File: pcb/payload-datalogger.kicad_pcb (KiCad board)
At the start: 2 copper layers, 43.5 x 41 mm, 42 parts, among them J1 2.54mm 01x02 header, J2 Conn_01x02, J3 Conn_01x02, J4 Conn_01x02, J5 Conn_01x02, SW2 PTS815, U1 XIAO-ESP32-C3-DIP, U2 NCP177AMX330TCG, U3 W25X40CLSN, U4 MCP96RL00T-E_MX, U5 MCP96RL00T-E_MX, U6 MCP96RL00T-E_MX, U7 MCP96RL00T-E_MX

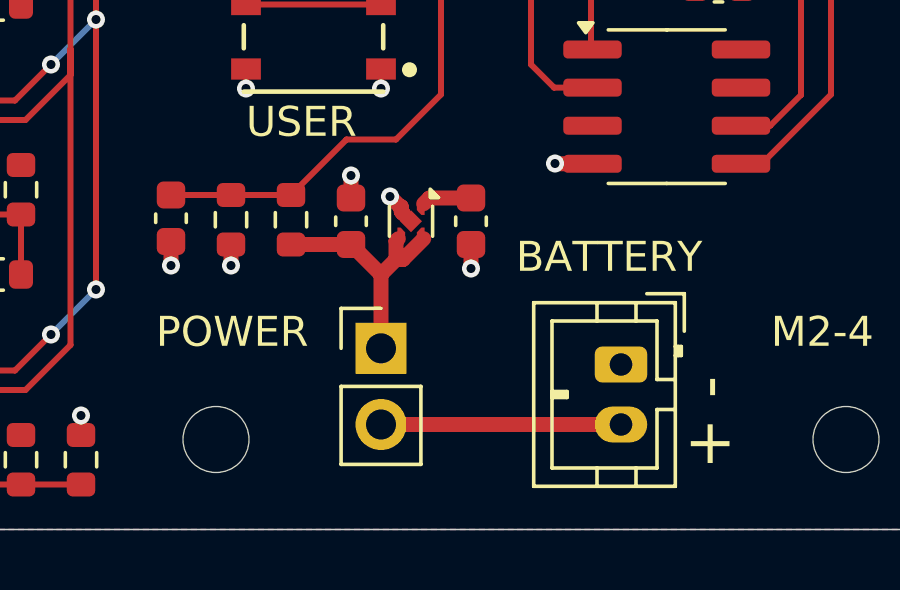
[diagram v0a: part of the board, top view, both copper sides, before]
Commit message: Update payload-datalogger.kicad_pcb
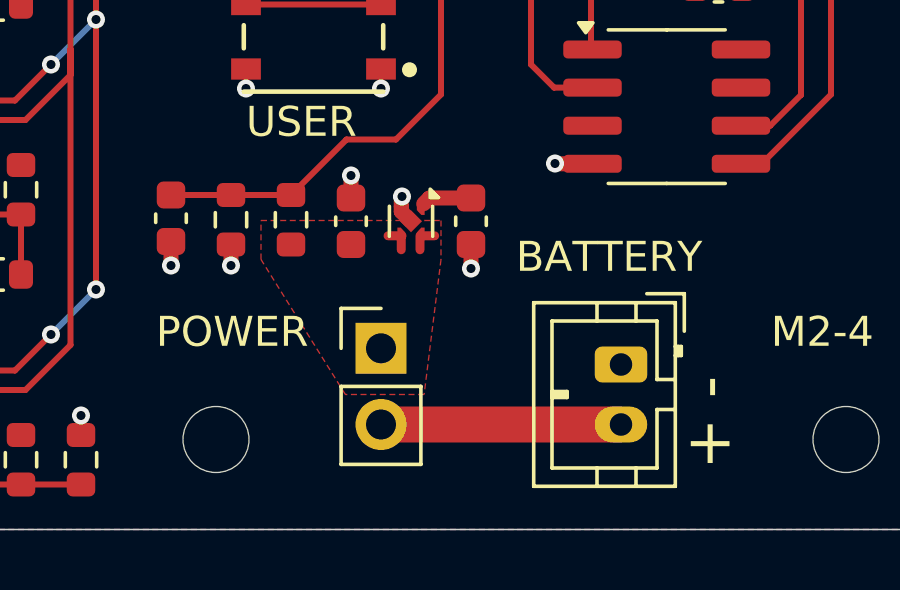
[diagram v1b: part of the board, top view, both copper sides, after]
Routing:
- net +BATT: track 8.52 -> 1.86 mm
- added copper zone on F.Cu, net +BATT
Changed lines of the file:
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@@
 		(start 104.5 76.5)
 		(end 96.5 76.5)
-		(width 0.5)
+		(width 1.2)
 		(layer "F.Cu")
 		(net 1)
@@
 	)
 	(segment
+		(start 97.175 68.925)
+		(end 97.2 68.9)
+		(width 0.5)
+		(layer "F.Cu")
+		(net 2)
+	)
+	(segment
 		(start 106.205 61.905)
 		(end 106.2 61.9)
@@
 	)
 	(segment
+		(start 97.5 69.725)
+		(end 97.175 69.4)
+		(width 0.5)
+		(layer "F.Cu")
+		(net 2)
+	)
+	(segment
 		(start 79.35 57.35)
 		(end 80 58)
@@
 	)
 	(segment
-		(start 97.175 69.4)
-		(end 97.239 69.464)
-		(width 0.5)
-		(layer "F.Cu")
-		(net 2)
-	)
-	(segment
 		(start 80 51.4375)
 		(end 80 50.375)
@@
 	)
 	(segment
-		(start 97.239 69.464)
-		(end 97.239 69.479)
-		(width 0.5)
-		(layer "F.Cu")
-		(net 2)
-	)
-	(segment
 		(start 81.3 65.7)
 		(end 80 67)
@@
 	)
 	(segment
-		(start 97.175 69.24)
-		(end 97.14 69.24)
-		(width 0.5)
-		(layer "F.Cu")
-		(net 2)
-	)
-	(segment
 		(start 79.35 66.35)
 		(end 80 67)
@@
 	)
 	(segment
-		(start 97.175 69.24)
-		(end 97.175 69.4)
-		(width 0.5)
-		(layer "F.Cu")
-		(net 2)
-	)
-	(segment
 		(start 82.4375 49)
 		(end 80 49)
@@
 	)
 	(segment
-		(start 97.14 69.24)
-		(end 96.8 68.9)
-		(width 0.5)
-		(layer "F.Cu")
-		(net 2)
-	)
-	(segment
 		(start 77.5625 47.7)
 		(end 78.7 47.7)
@@
 	)
 	(segment
+		(start 97.175 69.4)
+		(end 97.175 69.24)
+		(width 0.5)
+		(layer "F.Cu")
+		(net 2)
+	)
+	(segment
 		(start 96.500002 64.649998)
 		(end 96.500002 65.299998)
@@
 	)
 	(segment
+		(start 97.175 69.24)
+		(end 97.175 68.925)
+		(width 0.5)
+		(layer "F.Cu")
+		(net 2)
+	)
+	(segment
 		(start 77.5625 68.3)
 		(end 78.55 68.3)
@@
 	)
 	(via
-		(at 96.8 68.9)
-		(size 0.6)
-		(drill 0.3)
-		(layers "F.Cu" "B.Cu")
-		(net 2)
-	)
-	(via
 		(at 102.3 67.8)
 		(size 0.6)
@@
 	(via
 		(at 92 65.3)
+		(size 0.6)
+		(drill 0.3)
+		(layers "F.Cu" "B.Cu")
+		(net 2)
+	)
+	(via
+		(at 97.2 68.9)
 		(size 0.6)
 		(drill 0.3)
@@
 	)
 	(segment
-		(start 96.5 71.5)
-		(end 95.5 70.5)
-		(width 0.5)
+		(start 97.175 70.21)
+		(end 97.175 70.675)
+		(width 0.3)
 		(layer "F.Cu")
 		(net 5)
 	)
 	(segment
-		(start 97 71)
-		(end 97.230508 71)
-		(width 0.5)
+		(start 97.825 70.21)
+		(end 98.29 70.21)
+		(width 0.3)
 		(layer "F.Cu")
 		(net 5)
 	)
 	(segment
-		(start 97 71)
-		(end 97 70.385)
-		(width 0.5)
+		(start 97.8 70.21)
+		(end 97.8 70.675)
+		(width 0.3)
 		(layer "F.Cu")
 		(net 5)
 	)
 	(segment
-		(start 96.5 73.96)
-		(end 96.5 71.5)
-		(width 0.5)
-		(layer "F.Cu")
-		(net 5)
-	)
-	(segment
-		(start 97 70.385)
-		(end 97.077246 70.307754)
-		(width 0.5)
-		(layer "F.Cu")
-		(net 5)
-	)
-	(segment
-		(start 96.5 71.5)
-		(end 97 71)
-		(width 0.5)
-		(layer "F.Cu")
-		(net 5)
-	)
-	(segment
-		(start 97.230508 71)
-		(end 97.922754 70.307754)
-		(width 0.5)
-		(layer "F.Cu")
-		(net 5)
-	)
-	(segment
-		(start 95.5 70.5)
-		(end 93.5 70.5)
-		(width 0.5)
+		(start 97.2 70.21)
+		(end 96.735 70.21)
+		(width 0.3)
 		(layer "F.Cu")
 		(net 5)
@@
 			)
 		)
+	)
+	(zone
+		(net 5)
+		(net_name "+BATT")
+		(layer "F.Cu")
+		(hatch edge 0.5)
+		(priority 2)
+		(connect_pads
+			(clearance 0.2)
+		)
+		(min_thickness 0.2)
+		(filled_areas_thickness no)
+		(fill yes
+			(thermal_gap 0.2)
+			(thermal_bridge_width 0.5)
+		)
+		(polygon
+			(pts
+				(xy 95.3125 75.5) (xy 92.5 71) (xy 92.5 69.7) (xy 98.5 69.7) (xy 98.5 71) (xy 97.9375 75.5)
+			)
+		)
